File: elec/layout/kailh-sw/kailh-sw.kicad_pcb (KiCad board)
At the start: 2 copper layers, 4 parts, among them U1 100nF ±10% 16V X7R, U3 10kΩ ±1% 62.5mW

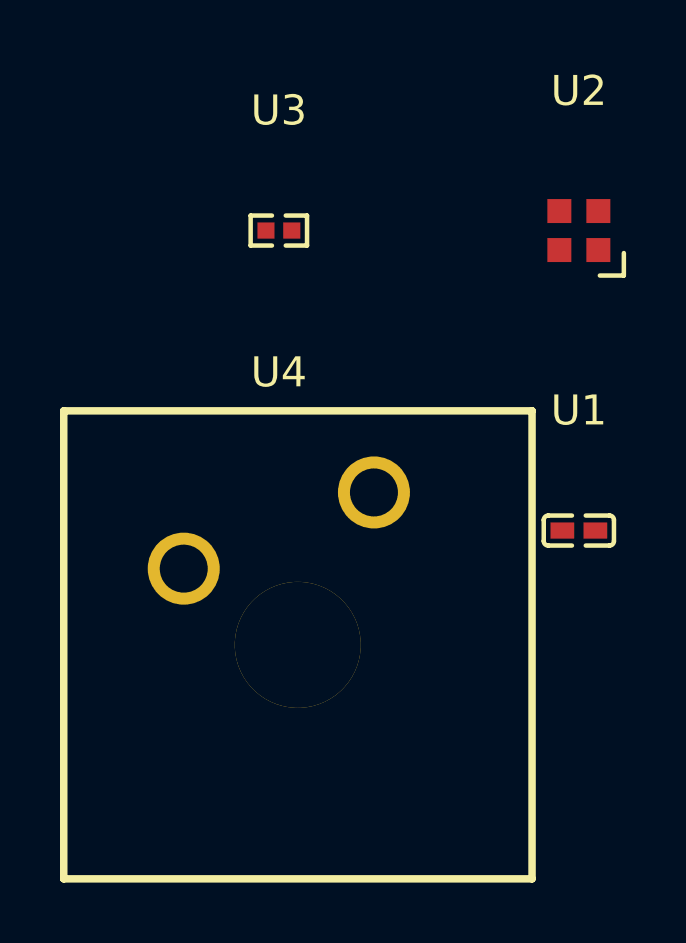
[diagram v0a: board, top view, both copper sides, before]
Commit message: build with v3
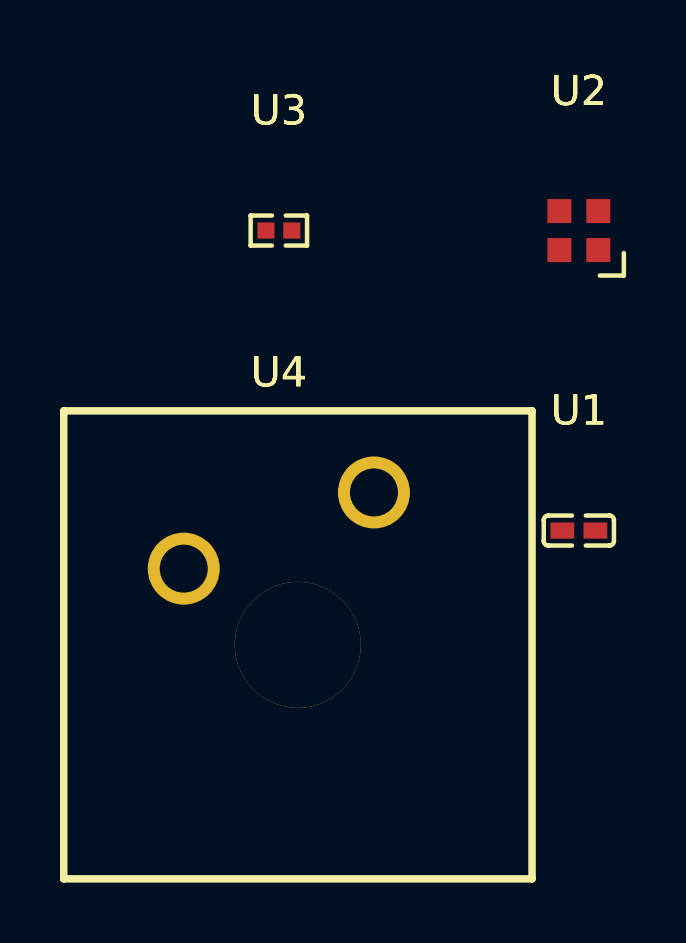
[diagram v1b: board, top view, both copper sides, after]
